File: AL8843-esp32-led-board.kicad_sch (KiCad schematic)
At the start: 11 parts, among them IC1 AL8843QSP-13

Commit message: jlcpcb order W2025081219518153
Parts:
- R1, R2: footprint Resistor_SMD:R_1206_3216Metric -> Resistor_SMD:R_2512_6332Metric; LCSC (none) -> C419755
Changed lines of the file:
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@@
 			)
 		)
-		(property "Footprint" "Resistor_SMD:R_1206_3216Metric"
+		(property "Footprint" "Resistor_SMD:R_2512_6332Metric"
 			(at 107.95 34.798 90)
 			(effects
@@
 		(property "Description" "Resistor"
 			(at 107.95 33.02 0)
+			(effects
+				(font
+					(size 1.27 1.27)
+				)
+				(hide yes)
+			)
+		)
+		(property "LCSC" "C419755"
+			(at 107.95 33.02 90)
 			(effects
 				(font
@@
 			)
 		)
-		(property "Footprint" "Resistor_SMD:R_1206_3216Metric"
+		(property "Footprint" "Resistor_SMD:R_2512_6332Metric"
 			(at 107.95 27.178 90)
 			(effects
@@
 			(effects
 				(font
+					(size 1.27 1.27)
+				)
+				(hide yes)
+			)
+		)
+		(property "LCSC" "C419755"
+			(at 107.95 25.4 90)
+			(effects
+				(font

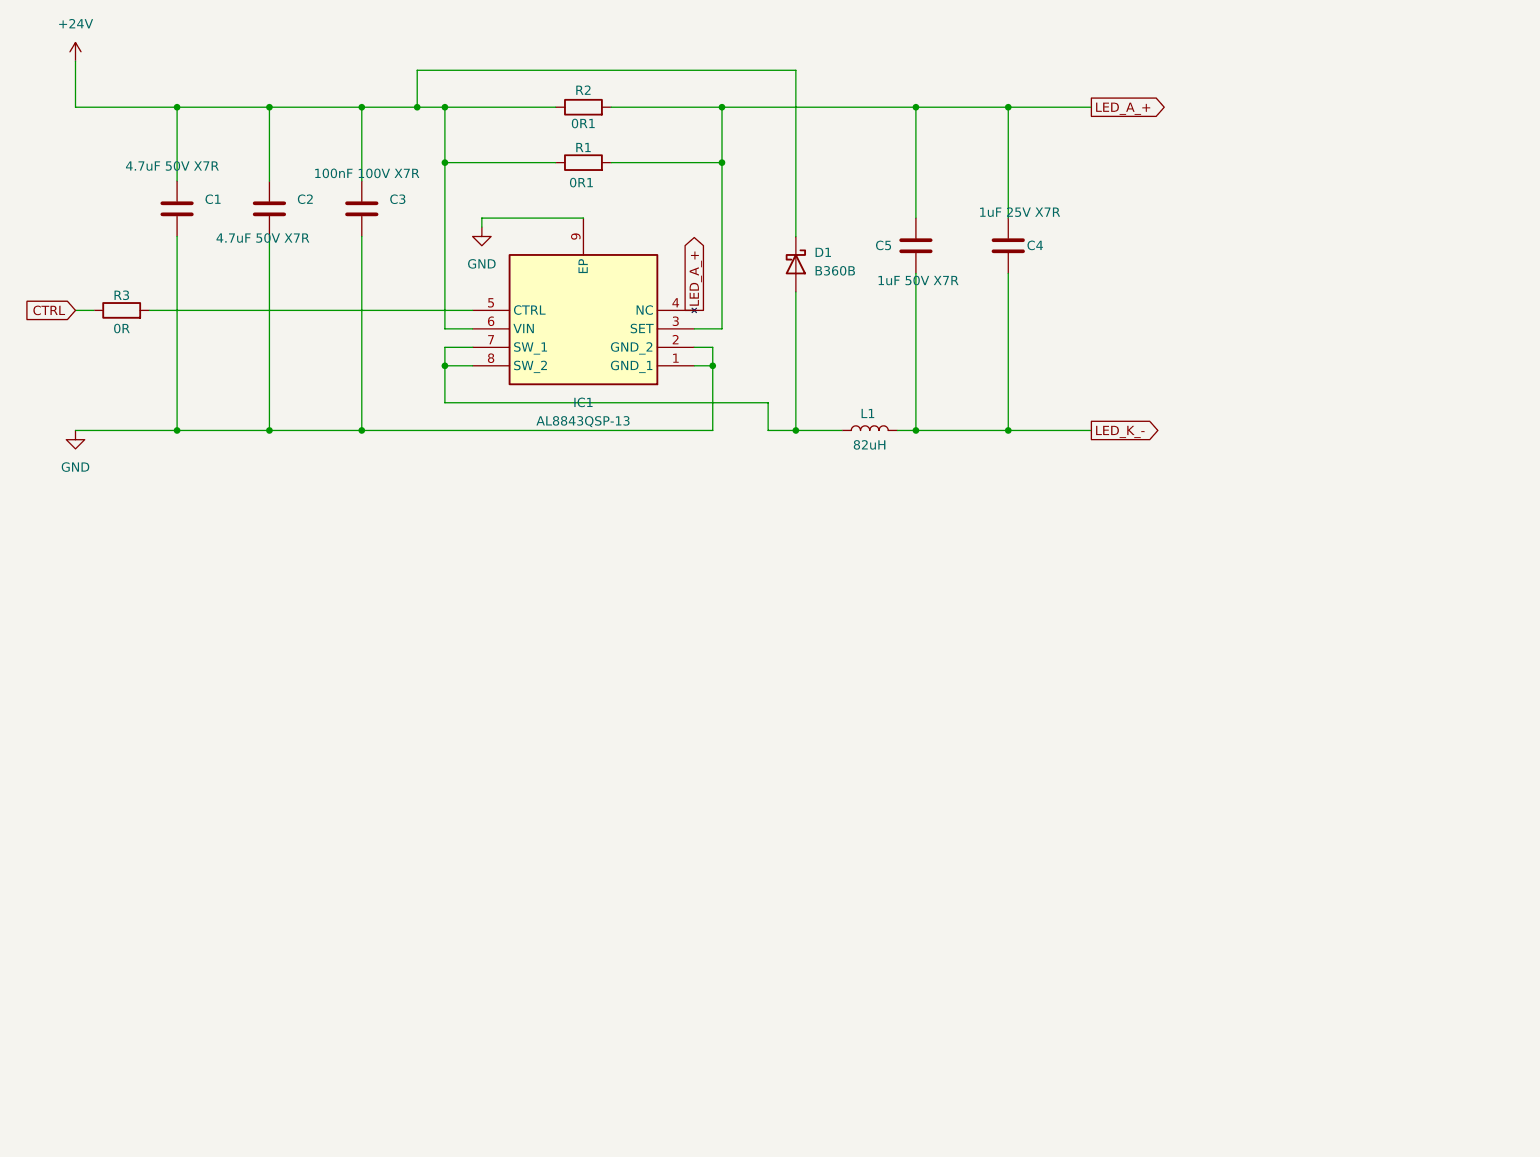
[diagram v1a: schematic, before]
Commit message: ESP32 power
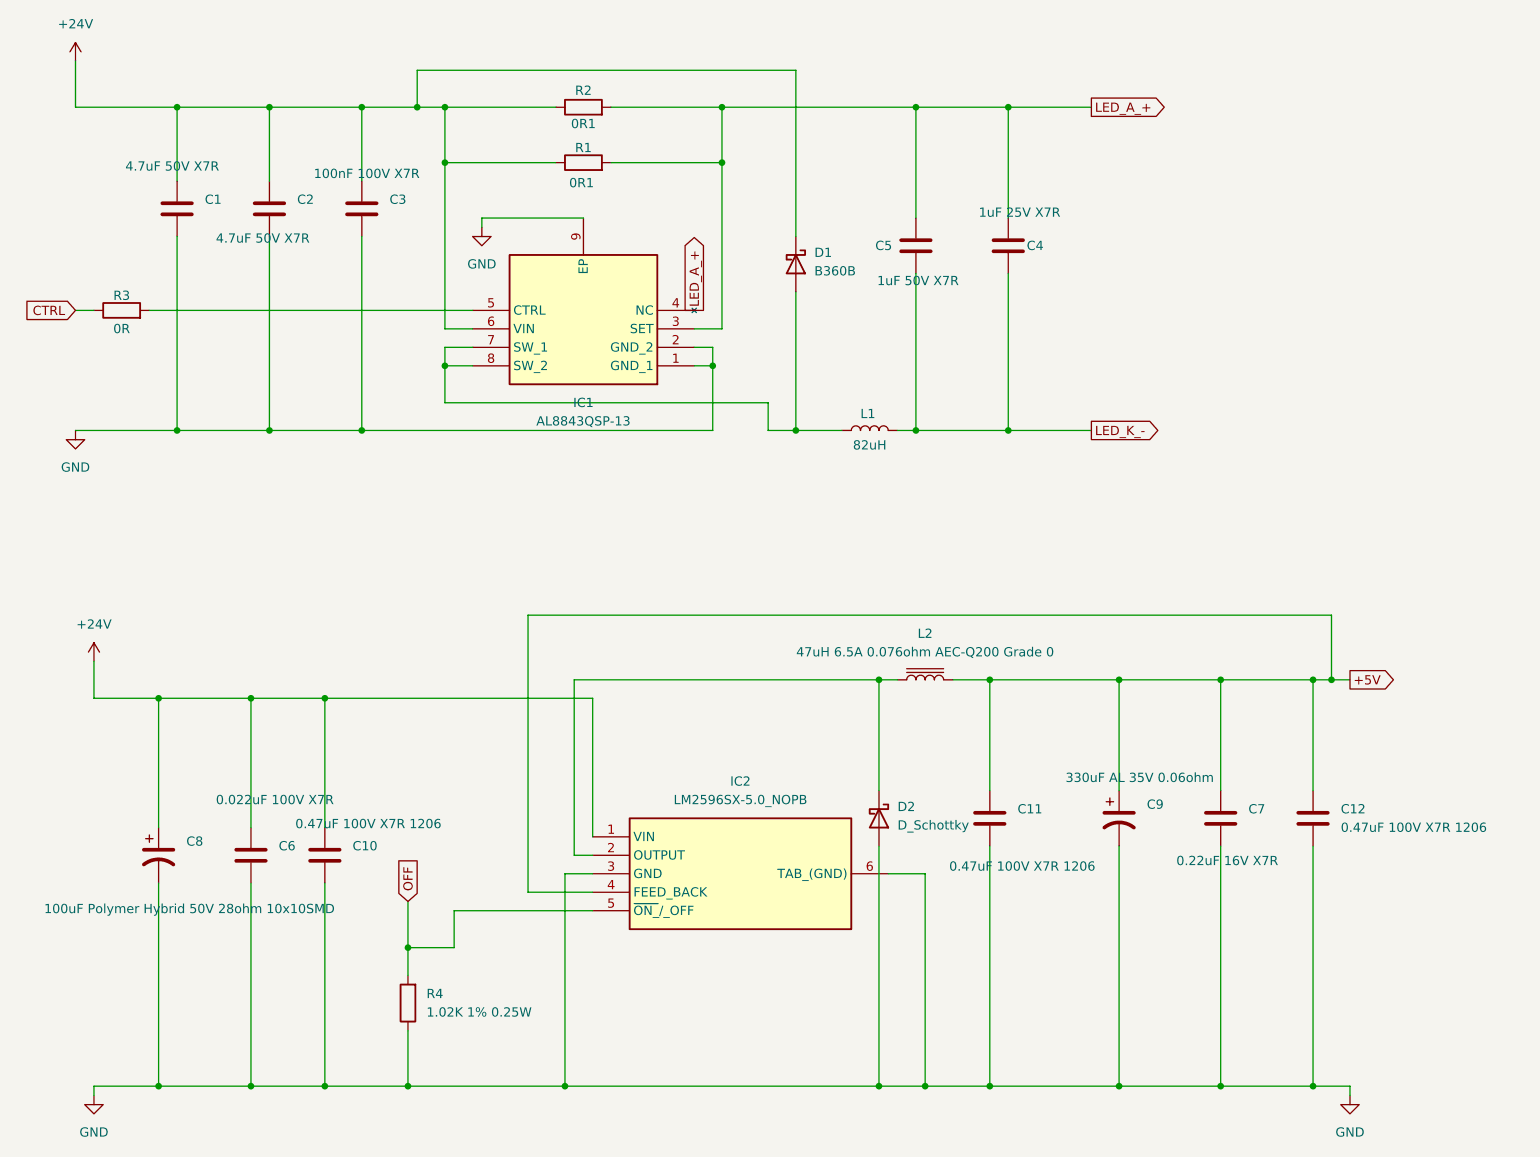
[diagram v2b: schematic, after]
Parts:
- added C10, C11, C12: 0.47uF 100V X7R 1206, Capacitor_SMD:C_1206_3216Metric, symbol Device:C
- added C6: 0.022uF 100V X7R, Capacitor_SMD:C_0603_1608Metric, symbol Device:C
- added C7: 0.22uF 16V X7R, Capacitor_SMD:C_0402_1005Metric, symbol Device:C
- added C8: 100uF Polymer Hybrid 50V 28ohm 10x10SMD, Capacitor_SMD:C_Elec_10x10.2, symbol Device:C_Polarized_US
- added C9: 330uF AL 35V 0.06ohm, Capacitor_SMD:CP_Elec_8x10, symbol Device:C_Polarized_US
- added D2: D_Schottky, Diode_SMD:D_SMC, symbol Device:D_Schottky
- added IC2: LM2596SX-5.0_NOPB, LM2596SX-5.0:KTT0005B, symbol LM2596SX-5_0_NOPB:LM2596SX-5.0_NOPB
- added L2: 47uH 6.5A 0.076ohm AEC-Q200 Grade 0, Inductor_SMD:L_TechFuse_SL1265, symbol Device:L_Iron
- added R4: 1.02K 1% 0.25W, Resistor_SMD:R_1206_3216Metric, symbol Device:R
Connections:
- net +24V: now also C10.1, C6.1, C8.1, IC2.1 (VIN)
- net GND: now also C10.2, C11.2, C12.2, C6.2, C7.2, C8.2, C9.2, D2.2 (A), IC2.3 (GND), IC2.6 (TAB_(GND)), R4.1
- new net: D2.1 (K), IC2.2 (OUTPUT), L2.1
- new net +5V: C11.1, C12.1, C7.1, C9.1, IC2.4 (FEED_BACK), L2.2
- new net OFF: IC2.5 (~{ON_}/_OFF), R4.2
